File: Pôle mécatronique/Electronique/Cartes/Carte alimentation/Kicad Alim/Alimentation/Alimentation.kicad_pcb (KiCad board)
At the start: 2 copper layers, 71.1 x 66 mm, 13 parts, among them J1 Conn_01x04, J2 Conn_01x04, J3 Conn_01x04, J4 Conn_01x05, J5 Conn_02x03_Odd_Even, J6 Conn_01x05, J7 Conn_02x10_Odd_Even, K1 G5LE-1, Q1 BSS138, U1 TSR_2-2450, U2 TSR_2-2450, U3 TSR_2-24120

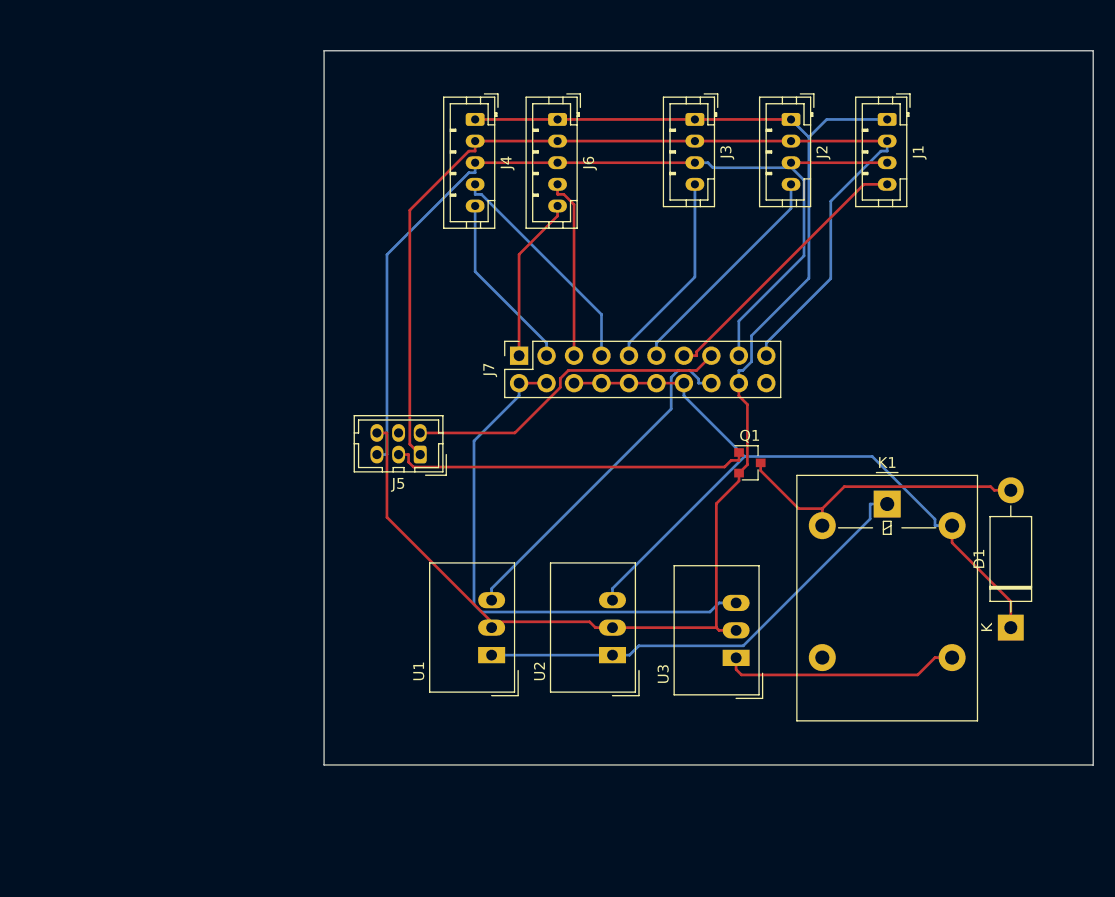
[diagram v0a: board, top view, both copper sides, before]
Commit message: Update alim
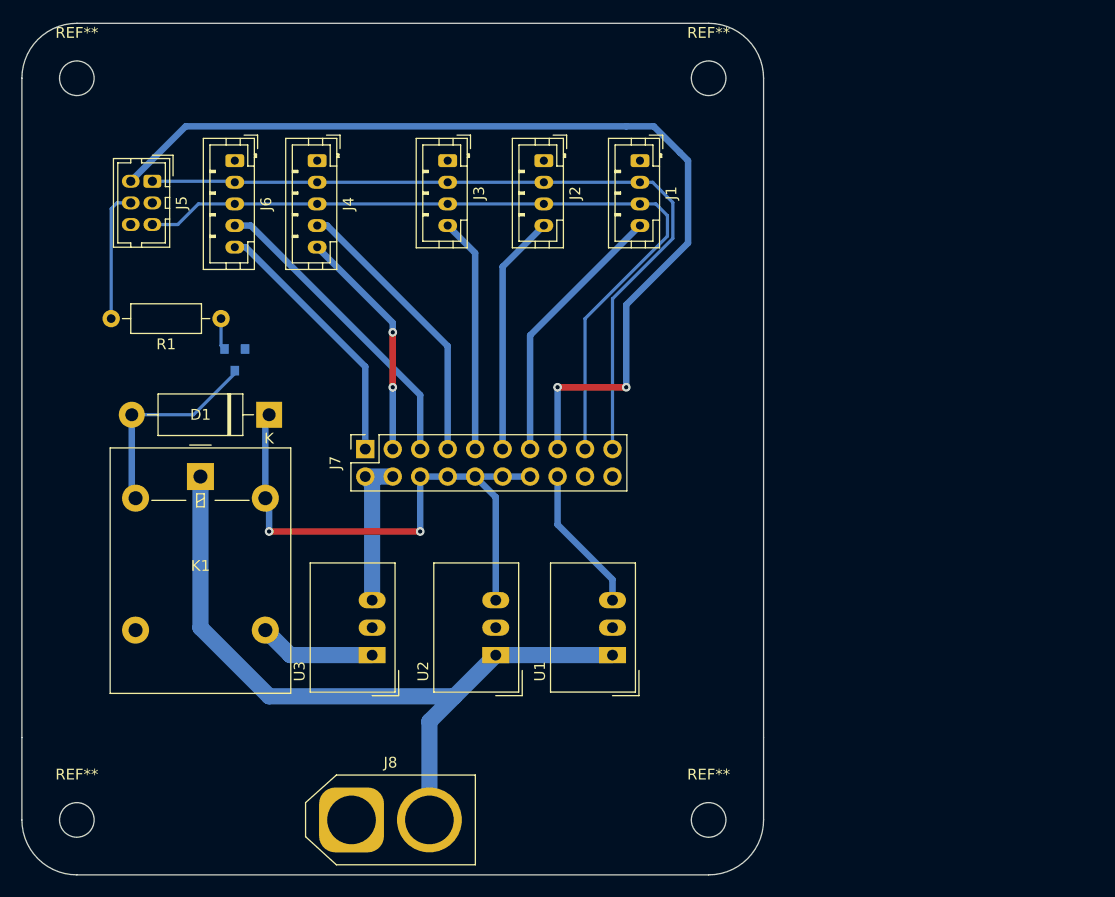
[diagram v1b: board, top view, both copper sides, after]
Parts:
- added J8: Conn_01x02, Connector_AMASS:AMASS_XT60-F_1x02_P7.20mm_Vertical, F.Cu at (116.3, 107.2)
- added R1: 6000, Resistor_THT:R_Axial_DIN0207_L6.3mm_D2.5mm_P10.16mm_Horizontal, F.Cu at (104.3, 60.8)
- added REF**: MountingHole_3.2mm_M3, MountingHole:MountingHole_3.2mm_M3, F.Cu at (90.9, 107.2)
- added REF**: MountingHole_3.2mm_M3, MountingHole:MountingHole_3.2mm_M3, F.Cu at (149.4, 107.2)
- added REF**: MountingHole_3.2mm_M3, MountingHole:MountingHole_3.2mm_M3, F.Cu at (90.9, 38.6)
- added REF**: MountingHole_3.2mm_M3, MountingHole:MountingHole_3.2mm_M3, F.Cu at (149.4, 38.6)
- Q1: moved to B.Cu
- moved D1 71.3 mm to (108.7, 69.7), turned to 180 degrees
- moved K1 63.6 mm to (102.4, 75.4)
- moved Q1 48.6 mm to (105.5, 64.6), turned to 270 degrees
- moved J5 35.4 mm to (97.9, 48.1), turned to 270 degrees
- moved U3 33.7 mm to (118.2, 91.9)
- moved J6 30.1 mm to (105.5, 46.2)
- moved J2 23.2 mm to (134.1, 46.2)
- moved J3 23.2 mm to (125.2, 46.2)
- moved J1 23.2 mm to (143.0, 46.2)
- moved J7 16.6 mm to (117.6, 72.9)
- moved J4 15.1 mm to (113.2, 46.2)
- moved U1 11.2 mm to (140.5, 91.9)
- moved U2 10.8 mm to (129.7, 91.9)
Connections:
- J5 pad 3: cmd_relais -> Net-(J5-Pad3)
- J5 pad 4: Net-(J5-Pad4) -> cmd_relais
- Q1 pad 1: cmd_relais -> Net-(Q1-Pad1)
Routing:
- net GND: track 135.1 -> 0.00 mm
- net 5VRPI: track 30.4 -> 90.3 mm, vias 0 -> 2
- net Net-(J7-Pad2): track 49.6 -> 14.2 mm
- net Vbatt: track 43.2 -> 69.1 mm
- net cmd_relais: track 33.3 -> 12.2 mm
- net can_H: track 95.1 -> 74.7 mm
- net 5V: track 71.5 -> 52.5 mm, vias 0 -> 2
- net Net-(J7-Pad16): track 32.2 -> 13.5 mm
- net can_L: track 90.8 -> 74.2 mm
- net 5Vout5: track 16.8 -> 28.6 mm
- net VbattProtected: track 21.9 -> 10.8 mm
- net 12Vout2: track 15.3 -> 24.3 mm
- net Net-(D1-Pad2): track 27.9 -> 19.2 mm
- net 5Vout4: track 21.0 -> 26.2 mm
- net 12Vout1: track 16.6 -> 21.6 mm, vias 0 -> 2
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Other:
- board size 71.1 x 66 mm -> 68.6 x 78.7 mm
